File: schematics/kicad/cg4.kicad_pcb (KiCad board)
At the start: 4 copper layers, 228 x 195.5 mm, 139 parts, among them J7 DE15_Socket_HighDensity, K1300 10uF, P4 DIN41612_03x32_C_Split, U1000 PAL16R8, U1001 PAL20X10, U1002 PAL20X10, U1003 PAL20X10, U1004 PAL20R6, U1005 P16L8, U1006 PAL16R8, U1007 P20L8, U1008 P16L8, U1009 P16L8, U1010 P16L8, U1015 74F175, U1016 74F244, U1017 330Ω, U1021 330Ω, U1036 330Ω, U1037 330Ω, U1038 330Ω, U1100 74F257, U1101 74F257, U1102 74F257, U1103 74F257, U1104 330Ω, U1105 330Ω, U1110 74F257, U1111 74F257, U1112 74F257, U1113 74F257, U1114 330Ω, U1129 74LS393, U1200 HM53461, U1201 HM53461, U1202 HM53461, U1203 HM53461, U1204 HM53461, U1205 HM53461, U1206 HM53461, U1207 HM53461, U1208 HM53461, U1209 HM53461, U1210 HM53461, U1211 HM53461, U1212 HM53461, U1213 HM53461, U1214 HM53461, U1215 HM53461, U1216 HM53461, U1217 HM53461, U1218 HM53461, U1219 HM53461, U1220 HM53461, U1221 HM53461, U1222 HM53461, U1223 HM53461, U1224 HM53461, U1225 HM53461, U1226 HM53461, U1227 HM53461, U1228 HM53461, U1229 HM53461, U1230 HM53461, U1231 HM53461, U1300 HM53461, U1301 HM53461, U1302 HM53461, U1303 HM53461, U1304 HM53461, U1305 HM53461, U1306 HM53461, U1307 HM53461, U1310 BT458, U1311 92.9405Mhz, U1312 10H101, U1313 10H131, U1314 10H350, U1315 LM385BZ-1.2, U1318 74F08

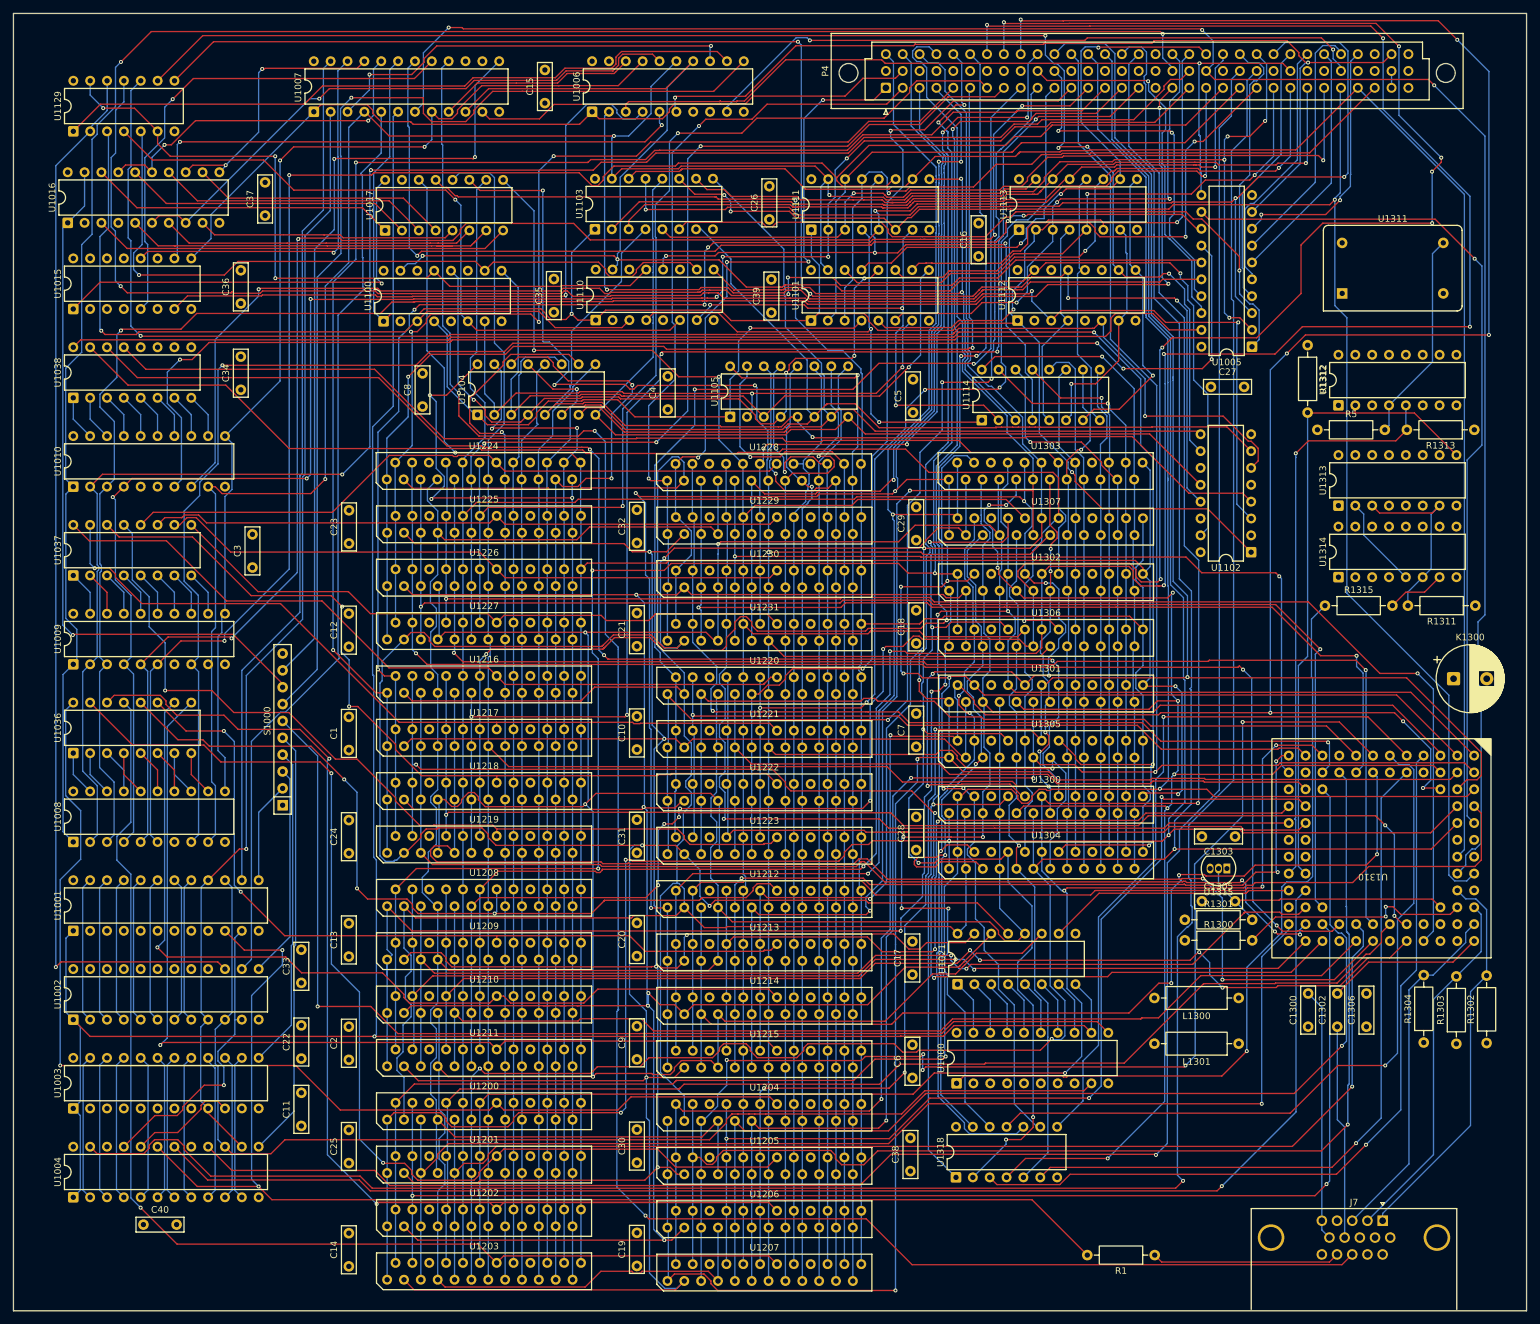
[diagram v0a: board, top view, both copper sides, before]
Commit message: Clean up
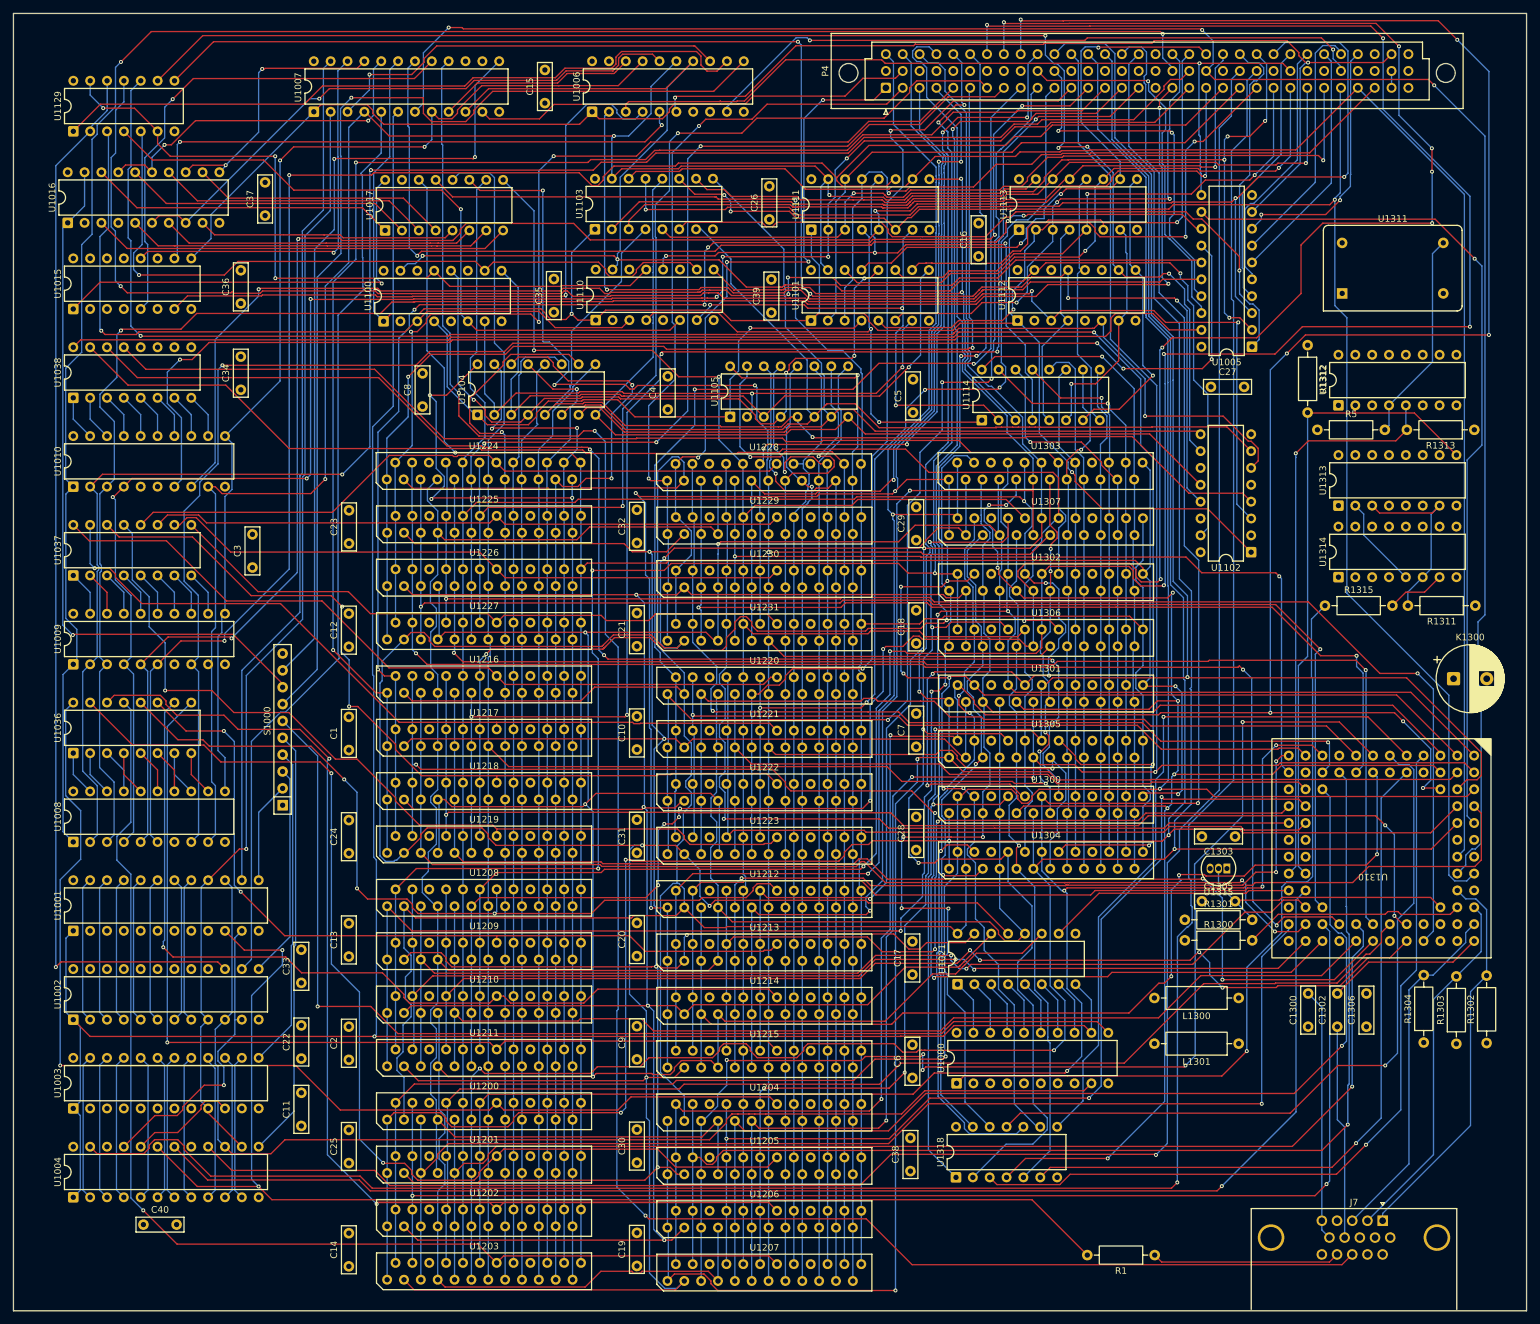
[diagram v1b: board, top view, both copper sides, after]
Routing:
- net /Video Output/V.D.D9: track 115.0 -> 105.0 mm
- net /Video Output/V.C.D6: track 189.5 -> 180.8 mm
- net /Video Control/W.SE-2: track 380.9 -> 376.3 mm, vias 5 -> 4
- net /Misc/D21: track 248.0 -> 245.2 mm
- net /Video Output/V.A.D9: track 163.3 -> 165.9 mm, vias 6 -> 4
- net Net-(U1016-2Y3): track 58.6 -> 56.2 mm
- net /Video Output/V.A.D1: track 182.2 -> 179.8 mm
- net /Video Control/W.SC.1: track 468.3 -> 466.0 mm
- net /Video Control/W.RE-13: track 148.2 -> 146.2 mm
- net /Video Control/V.CNT: track 105.0 -> 106.8 mm
- net /Video Mux/W.1.A0: track 158.8 -> 157.0 mm
- net /Video Control/V.REF-: track 62.9 -> 61.4 mm, vias 2 -> 1
- net /Video Output/V.C.D3: track 114.6 -> 113.1 mm
- net /Misc/EN.VIDEO: track 343.8 -> 342.3 mm
- net Net-(U1310-FSA): track 34.8 -> 33.3 mm, vias 2 -> 0
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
